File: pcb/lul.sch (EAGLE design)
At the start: 88 parts, among them IC1 STM32F072C8T6, IC2 REG1117, IC3 74LVC1G125DBV, U1 UG-2864HSWEG01, X1 USB-MICROB

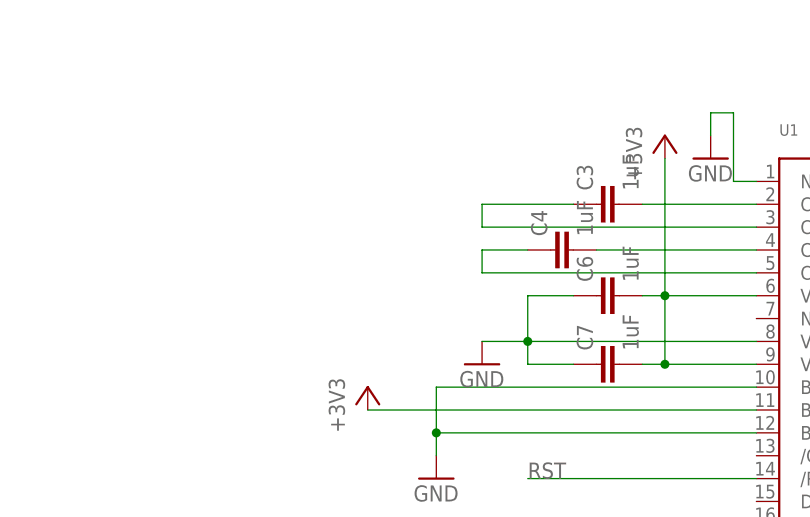
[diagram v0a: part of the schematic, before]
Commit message: RTOS working start
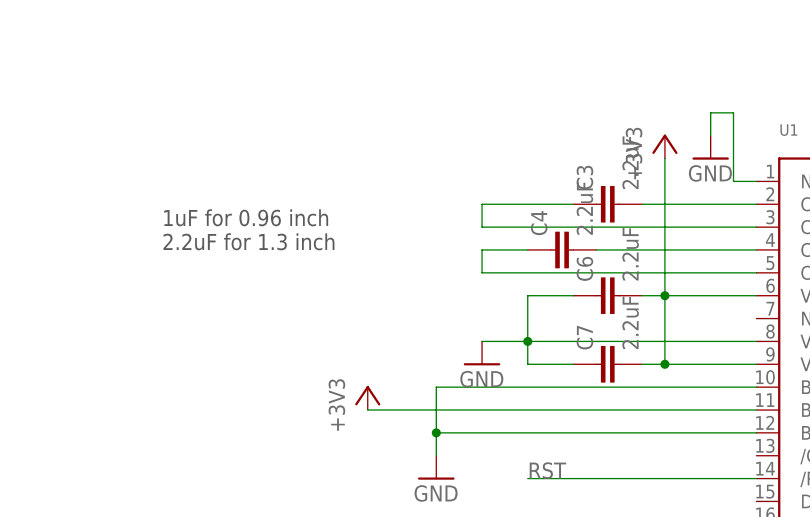
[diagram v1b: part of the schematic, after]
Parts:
- C3, C4, C6, C7: value 1uF -> 2.2uF
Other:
- note added: "1uF for 0.96 inch 2.2uF for 1.3 inch"
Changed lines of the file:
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@@
 <part name="U$2" library="supply1" library_urn="urn:adsk.eagle:library:371" deviceset="GND" device=""/>
 <part name="R3" library="clock" deviceset="RESISTOR" device="0805-RES" value="390K"/>
-<part name="C3" library="clock" deviceset="CAP" device="0805" value="1uF"/>
-<part name="C4" library="clock" deviceset="CAP" device="0805" value="1uF"/>
+<part name="C3" library="clock" deviceset="CAP" device="0805" value="2.2uF"/>
+<part name="C4" library="clock" deviceset="CAP" device="0805" value="2.2uF"/>
 <part name="U$18" library="supply1" library_urn="urn:adsk.eagle:library:371" deviceset="GND" device=""/>
 <part name="U$19" library="supply1" library_urn="urn:adsk.eagle:library:371" deviceset="GND" device=""/>
 <part name="C5" library="clock" deviceset="CAP" device="0805" value="10uF"/>
 <part name="U$20" library="supply1" library_urn="urn:adsk.eagle:library:371" deviceset="GND" device=""/>
-<part name="C7" library="clock" deviceset="CAP" device="0805" value="1uF"/>
+<part name="C7" library="clock" deviceset="CAP" device="0805" value="2.2uF"/>
 <part name="C8" library="clock" deviceset="CAP" device="0805" value="2.2uF/16V"/>
 <part name="U$21" library="supply1" library_urn="urn:adsk.eagle:library:371" deviceset="GND" device=""/>
-<part name="C6" library="clock" deviceset="CAP" device="0805" value="1uF"/>
+<part name="C6" library="clock" deviceset="CAP" device="0805" value="2.2uF"/>
 <part name="IC1" library="clock" deviceset="STM32F072C8T6" device=""/>
 <part name="SD1" library="clock" deviceset="TF-HOLDER" device=""/>
@@
 <sheet>
 <plain>
+<text x="297.18" y="63.5" size="1.778" layer="97">1uF for 0.96 inch
+2.2uF for 1.3 inch </text>
 </plain>
 <instances>
@@
 </drawing>
 <compatibility>
+<note version="6.3" minversion="6.2.2" severity="warning">
+Since Version 6.2.2 text objects can contain more than one line,
+which will not be processed correctly with this version.
+</note>
 <note version="8.2" severity="warning">
 Since Version 8.2, Eagle supports online libraries. The ids
